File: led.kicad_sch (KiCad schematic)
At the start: 11 parts, among them U4 C5944

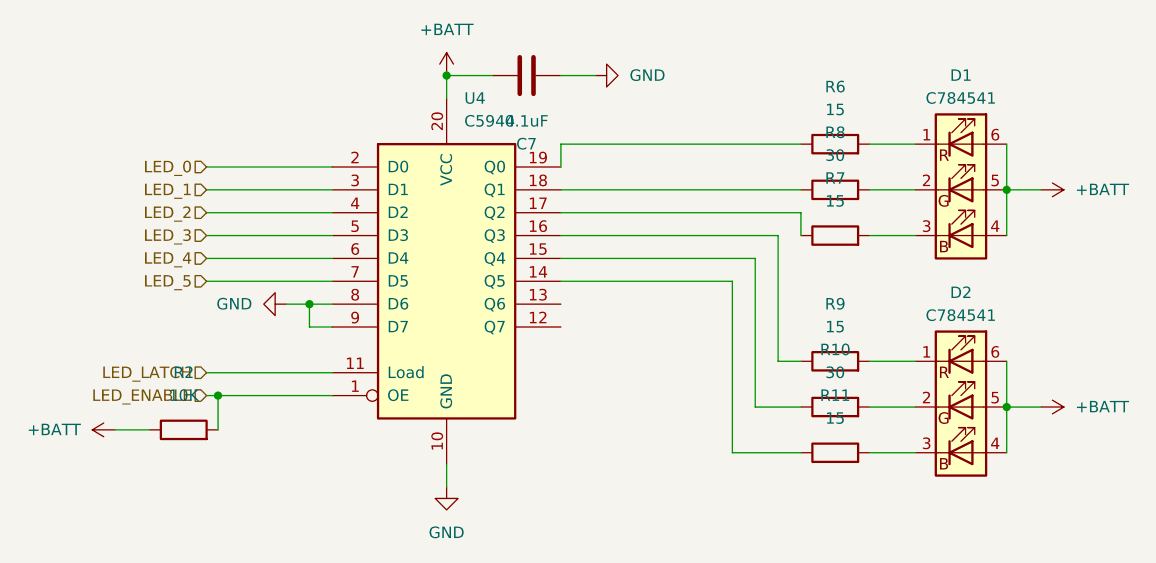
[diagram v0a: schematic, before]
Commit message: Field updates, generating fab files
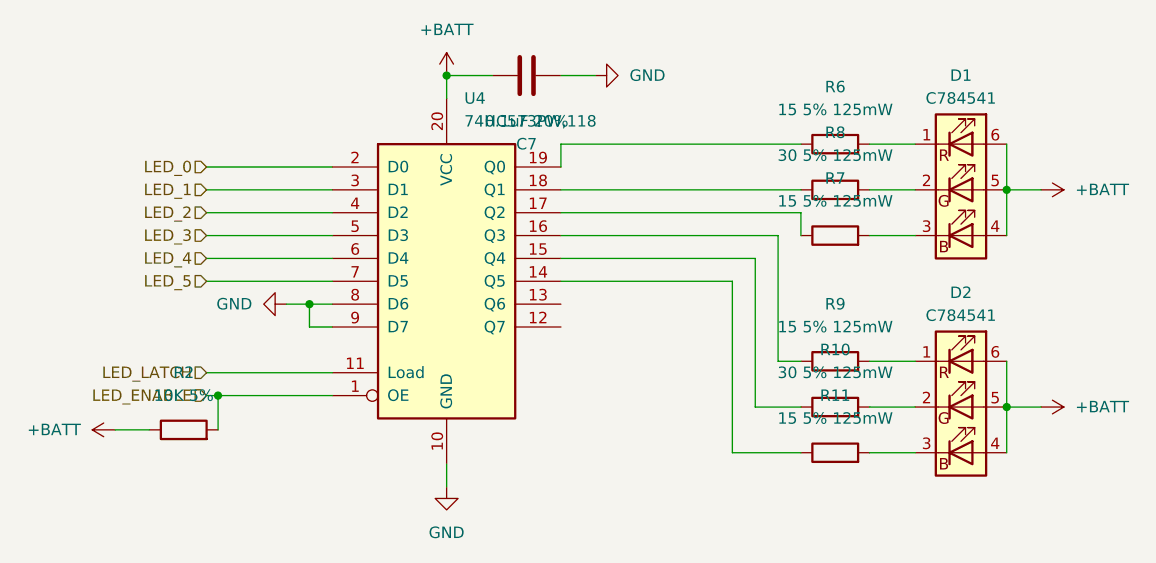
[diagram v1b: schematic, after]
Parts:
- C7: value 0.1uF -> 0.1uF 20%; JLCPCB Part # (none) -> C359190
- D1, D2: JLCPCB Part # (none) -> C784541
- R10, R8: value 30 -> 30 5% 125mW; JLCPCB Part # (none) -> C2930273
- R11, R6, R7, R9: value 15 -> 15 5% 125mW; JLCPCB Part # (none) -> C2930246
- R2: value 10K -> 10K 5%; JLCPCB Part # (none) -> C2906885
- U4: value C5944 -> 74HC573PW,118; JLCPCB Part # (none) -> C5944
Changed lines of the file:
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@@
       (effects (font (size 1.27 1.27)) (justify left))
     )
-    (property "Value" "C5944" (at 97.2059 69.85 0)
+    (property "Value" "74HC573PW,118" (at 97.2059 69.85 0)
       (effects (font (size 1.27 1.27)) (justify left))
     )
@@
     )
     (property "Datasheet" "74xx/74hc573.pdf" (at 95.25 87.63 0)
+      (effects (font (size 1.27 1.27)) hide)
+    )
+    (property "JLCPCB Part #" "C5944" (at 95.25 87.63 0)
       (effects (font (size 1.27 1.27)) hide)
     )
@@
       (effects (font (size 1.27 1.27)) hide)
     )
-    (property "Datasheet" "~" (at 152.4 102.87 0)
+    (property "Datasheet" "https://www.lcsc.com/product-detail/Light-Emitting-Diodes-LED_TCWIN-TC5050RGBF20-3CES-AF51_C784541.html" (at 152.4 102.87 0)
+      (effects (font (size 1.27 1.27)) hide)
+    )
+    (property "JLCPCB Part #" "C784541" (at 152.4 101.6 0)
       (effects (font (size 1.27 1.27)) hide)
     )
@@
       (effects (font (size 1.27 1.27)))
     )
-    (property "Value" "15" (at 138.43 78.74 90)
+    (property "Value" "15 5% 125mW" (at 138.43 78.74 90)
       (effects (font (size 1.27 1.27)))
     )
@@
       (effects (font (size 1.27 1.27)) hide)
     )
-    (property "Datasheet" "~" (at 138.43 82.55 0)
+    (property "Datasheet" "https://www.lcsc.com/product-detail/Chip-Resistor-Surface-Mount_FOJAN-FRC0805J150TS_C2930246.html" (at 138.43 82.55 0)
+      (effects (font (size 1.27 1.27)) hide)
+    )
+    (property "JLCPCB Part #" "C2930246" (at 138.43 82.55 0)
       (effects (font (size 1.27 1.27)) hide)
     )
@@
       (effects (font (size 1.27 1.27)))
     )
-    (property "Value" "30" (at 138.43 97.79 90)
+    (property "Value" "30 5% 125mW" (at 138.43 97.79 90)
       (effects (font (size 1.27 1.27)))
     )
@@
       (effects (font (size 1.27 1.27)) hide)
     )
-    (property "Datasheet" "~" (at 138.43 101.6 0)
+    (property "Datasheet" "https://www.lcsc.com/product-detail/Chip-Resistor-Surface-Mount_FOJAN-FRC0805J300TSD_C2930273.html" (at 138.43 101.6 0)
+      (effects (font (size 1.27 1.27)) hide)
+    )
+    (property "JLCPCB Part #" "C2930273" (at 138.43 101.6 0)
       (effects (font (size 1.27 1.27)) hide)
     )
@@
       (effects (font (size 1.27 1.27)))
     )
-    (property "Value" "0.1uF" (at 104.14 69.85 90)
+    (property "Value" "0.1uF 20%" (at 104.14 69.85 90)
       (effects (font (size 1.27 1.27)))
     )
@@
       (effects (font (size 1.27 1.27)) hide)
     )
-    (property "Datasheet" "~" (at 104.14 64.77 0)
+    (property "Datasheet" "https://www.lcsc.com/product-detail/Multilayer-Ceramic-Capacitors-MLCC-SMD-SMT_CCTC-TCC0402X5R104M250AT_C359190.html" (at 104.14 64.77 0)
+      (effects (font (size 1.27 1.27)) hide)
+    )
+    (property "JLCPCB Part #" "C359190" (at 104.14 64.77 0)
       (effects (font (size 1.27 1.27)) hide)
     )
@@
       (effects (font (size 1.27 1.27)) hide)
     )
-    (property "Datasheet" "~" (at 152.4 78.74 0)
+    (property "Datasheet" "https://www.lcsc.com/product-detail/Light-Emitting-Diodes-LED_TCWIN-TC5050RGBF20-3CES-AF51_C784541.html" (at 152.4 78.74 0)
+      (effects (font (size 1.27 1.27)) hide)
+    )
+    (property "JLCPCB Part #" "C784541" (at 152.4 77.47 0)
       (effects (font (size 1.27 1.27)) hide)
     )
@@
       (effects (font (size 1.27 1.27)))
     )
-    (property "Value" "30" (at 138.43 73.66 90)
+    (property "Value" "30 5% 125mW" (at 138.43 73.66 90)
       (effects (font (size 1.27 1.27)))
     )
@@
       (effects (font (size 1.27 1.27)) hide)
     )
-    (property "Datasheet" "~" (at 138.43 77.47 0)
+    (property "Datasheet" "https://www.lcsc.com/product-detail/Chip-Resistor-Surface-Mount_FOJAN-FRC0805J300TSD_C2930273.html" (at 138.43 77.47 0)
+      (effects (font (size 1.27 1.27)) hide)
+    )
+    (property "JLCPCB Part #" "C2930273" (at 138.43 77.47 0)
       (effects (font (size 1.27 1.27)) hide)
     )
@@
       (effects (font (size 1.27 1.27)))
     )
-    (property "Value" "15" (at 138.43 102.87 90)
+    (property "Value" "15 5% 125mW" (at 138.43 102.87 90)
       (effects (font (size 1.27 1.27)))
     )
@@
       (effects (font (size 1.27 1.27)) hide)
     )
-    (property "Datasheet" "~" (at 138.43 106.68 0)
+    (property "Datasheet" "https://www.lcsc.com/product-detail/Chip-Resistor-Surface-Mount_FOJAN-FRC0805J150TS_C2930246.html" (at 138.43 106.68 0)
+      (effects (font (size 1.27 1.27)) hide)
+    )
+    (property "JLCPCB Part #" "C2930246" (at 138.43 106.68 0)
       (effects (font (size 1.27 1.27)) hide)
     )
@@
       (effects (font (size 1.27 1.27)))
     )
-    (property "Value" "15" (at 138.43 68.58 90)
+    (property "Value" "15 5% 125mW" (at 138.43 68.58 90)
       (effects (font (size 1.27 1.27)))
     )
@@
       (effects (font (size 1.27 1.27)) hide)
     )
-    (property "Datasheet" "~" (at 138.43 72.39 0)
+    (property "Datasheet" "https://www.lcsc.com/product-detail/Chip-Resistor-Surface-Mount_FOJAN-FRC0805J150TS_C2930246.html" (at 138.43 72.39 0)
+      (effects (font (size 1.27 1.27)) hide)
+    )
+    (property "JLCPCB Part #" "C2930246" (at 138.43 72.39 0)
       (effects (font (size 1.27 1.27)) hide)
     )
@@
       (effects (font (size 1.27 1.27)))
     )
-    (property "Value" "15" (at 138.43 92.71 90)
+    (property "Value" "15 5% 125mW" (at 138.43 92.71 90)
       (effects (font (size 1.27 1.27)))
     )
@@
       (effects (font (size 1.27 1.27)) hide)
     )
-    (property "Datasheet" "~" (at 138.43 96.52 0)
+    (property "Datasheet" "https://www.lcsc.com/product-detail/Chip-Resistor-Surface-Mount_FOJAN-FRC0805J150TS_C2930246.html" (at 138.43 96.52 0)
+      (effects (font (size 1.27 1.27)) hide)
+    )
+    (property "JLCPCB Part #" "C2930246" (at 138.43 96.52 0)
       (effects (font (size 1.27 1.27)) hide)
     )
@@
       (effects (font (size 1.27 1.27)))
     )
-    (property "Value" "10K" (at 66.04 100.33 90)
+    (property "Value" "10K 5%" (at 66.04 100.33 90)
       (effects (font (size 1.27 1.27)))
     )
@@
       (effects (font (size 1.27 1.27)) hide)
     )
-    (property "Datasheet" "~" (at 66.04 104.14 0)
-      (effects (font (size 1.27 1.27)) hide)
-    )
+    (property "Datasheet" "https://www.lcsc.com/product-detail/Chip-Resistor-Surface-Mount_FOJAN-FRC0402J103-TS_C2906885.html" (at 66.04 104.14 0)
+      (effects (font (size 1.27 1.27)) hide)
+    )
+    (property "JLCPCB Part #" "C2906885" (at 66.04 104.14 0)
+      (effects (font (size 1.27 1.27)) hide)
+    )
